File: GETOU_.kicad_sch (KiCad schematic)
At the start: 13 parts

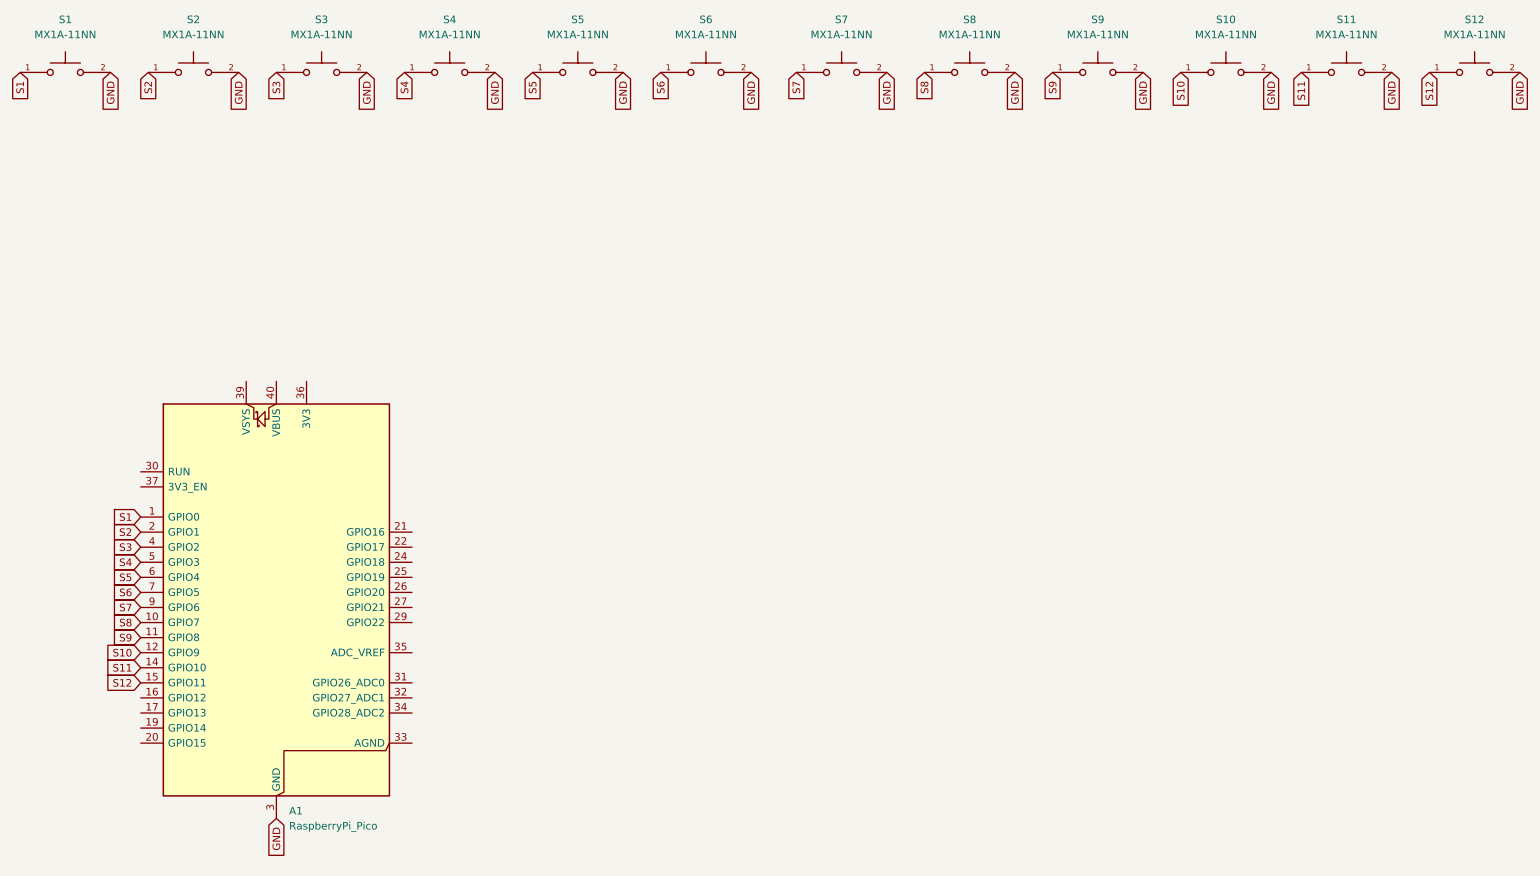
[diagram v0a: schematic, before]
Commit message: Modify PCB
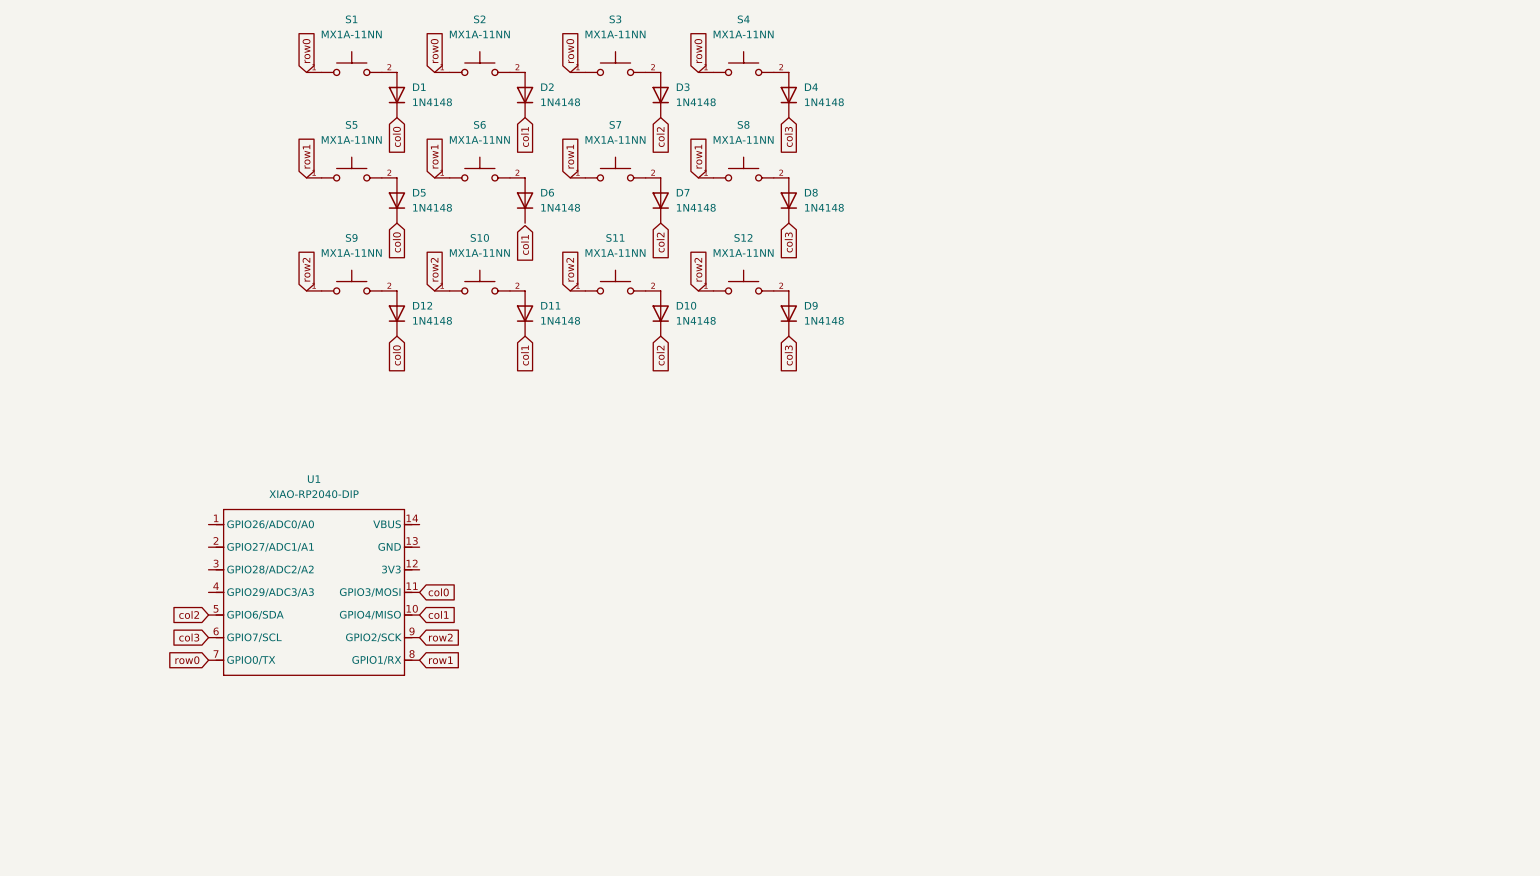
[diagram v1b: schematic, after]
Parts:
- removed A1: RaspberryPi_Pico, Module:RaspberryPi_Pico_Common_Unspecified, symbol MCU_Module:RaspberryPi_Pico
- added D1, D10, D11, D12, D2, D3, D4, D5, D6, D7, D8, D9: 1N4148, Diode_THT:D_DO-35_SOD27_P7.62mm_Horizontal, symbol Diode:1N4148
- added U1: XIAO-RP2040-DIP, footprints:XIAO-RP2040-DIP, symbol Seeed_Studio_XIAO_Series:XIAO-RP2040-DIP
- S1, S10, S11, S12, S2, S3, S4, S5, S6, S7, S8, S9: footprint MX1A-11NN:SW_MX1A-11NN -> footprints:SW_MX1A-11NN
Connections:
- net S11 is gone; now on net row2: S11.1
- net S12 is gone; now on net row2: S12.1
- net S2 is gone; now on net row0: S2.1
- net S3 is gone; now on net row0: S3.1
- net S4 is gone; now on net row0: S4.1
- net S6 is gone; now on net row1: S6.1
- net S7 is gone; now on net row1: S7.1
- net S8 is gone; now on net row1: S8.1
- net S9 is gone; now on net row2: S9.1
- removed net GND: S1.2, S10.2, S11.2, S12.2, S2.2, S3.2, S4.2, S5.2, S6.2, S7.2, S8.2, S9.2
- net S1 renamed row0
- net row0: now also U1.7 (GPIO0/TX)
- net S10 renamed row2
- net row2: now also U1.9 (GPIO2/SCK)
- net S5 renamed row1
- net row1: now also U1.8 (GPIO1/RX)
- new net: D11.2 (A), S10.2
- new net: D7.2 (A), S7.2
- new net: D12.2 (A), S9.2
- new net: D1.2 (A), S1.2
- new net: D4.2 (A), S4.2
- new net: D9.2 (A), S12.2
- new net: D8.2 (A), S8.2
- new net: D10.2 (A), S11.2
- new net: D6.2 (A), S6.2
- new net: D5.2 (A), S5.2
- new net: D3.2 (A), S3.2
- new net: D2.2 (A), S2.2
- new net col0: D1.1 (K), D12.1 (K), D5.1 (K), U1.11 (GPIO3/MOSI)
- new net col1: D11.1 (K), D2.1 (K), U1.10 (GPIO4/MISO)
- new net col2: D10.1 (K), D3.1 (K), D7.1 (K), U1.5 (GPIO6/SDA)
- new net col3: D4.1 (K), D8.1 (K), D9.1 (K), U1.6 (GPIO7/SCL)
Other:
- moved on the sheet: S1, S10, S11, S12, S2, S3, S4, S5, S6, S7, S8, S9
